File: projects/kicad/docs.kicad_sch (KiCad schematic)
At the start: 20 parts, among them J1 Micro_SD_Card, SW1 SW_PUSH, SW2 SW_PUSH, SW3 SW_PUSH, SW4 SW_PUSH, SW5 SW_PUSH, SW6 SW_PUSH, SW7 RotaryEncoder_Switch, U1 Pico, U2 LCD

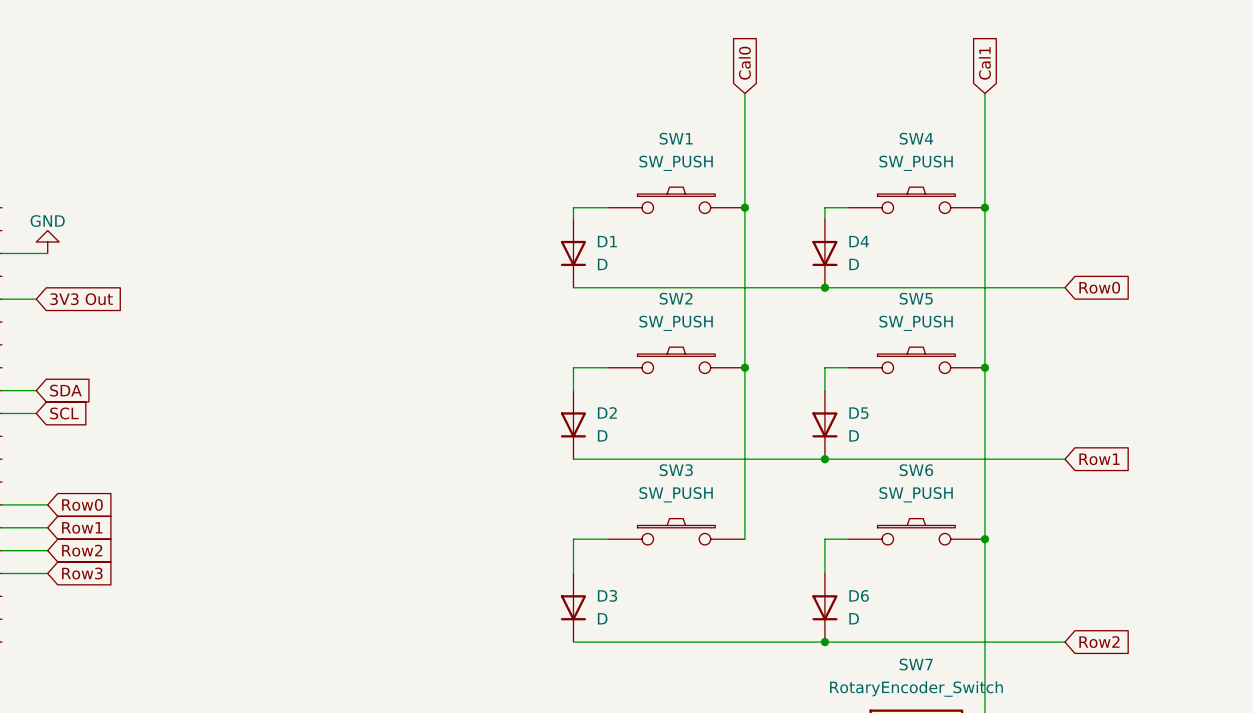
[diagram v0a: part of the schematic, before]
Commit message: Update_0122
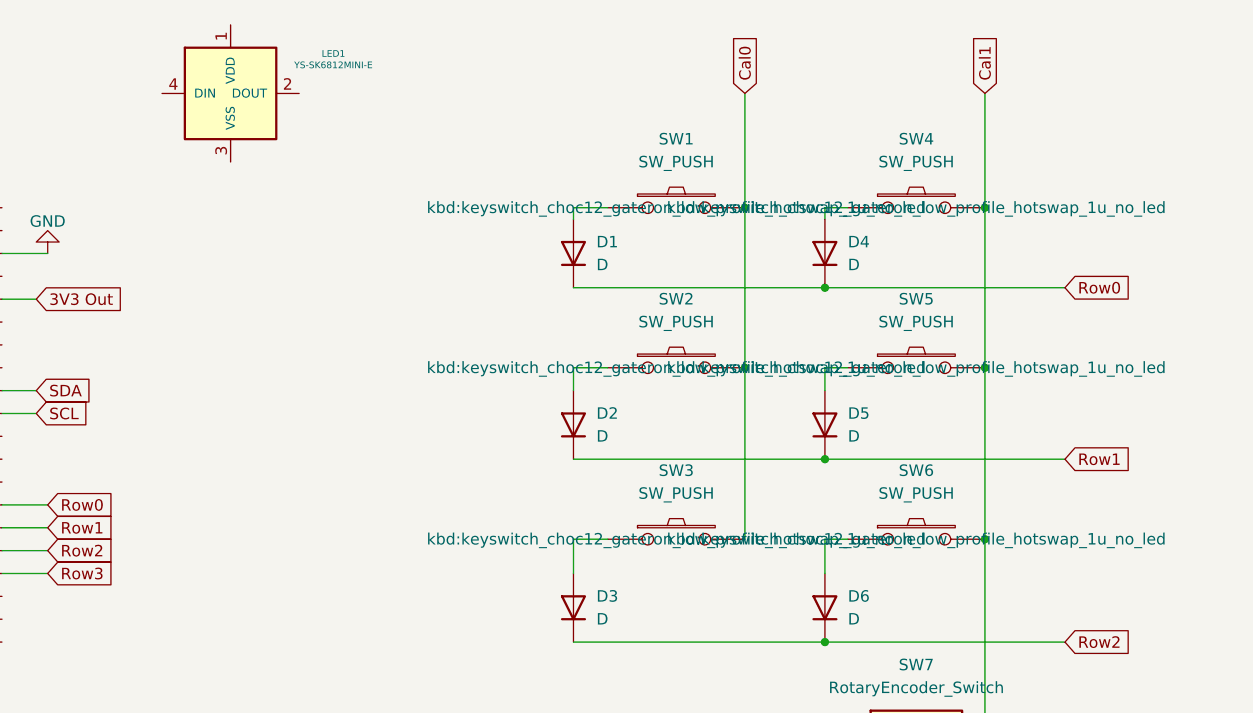
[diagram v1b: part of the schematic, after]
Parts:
- added LED1: YS-SK6812MINI-E, symbol kbd:YS-SK6812MINI-E
- D1, D2, D3, D4, D5, D6, D7: footprint (none) -> kbd_parts:D_SOD-123-Pretty
- SW1, SW2, SW3, SW4, SW5, SW6: footprint (none) -> kbd:keyswitch_choc12_gateron_low_profile_hotswap_1u_no_led
- SW7: footprint (none) -> Rotary_Encoder:RotaryEncoder_Bourns_Vertical_PEC12R-3x17F-Sxxxx
- U2: footprint (none) -> ST7789v_Library:ST7789V
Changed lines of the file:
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@@
 			)
 		)
-		(property "Footprint" ""
+		(property "Footprint" "kbd:keyswitch_choc12_gateron_low_profile_hotswap_1u_no_led"
 			(at 177.8 39.37 0)
 			(effects
@@
 			)
 		)
-		(property "Footprint" ""
+		(property "Footprint" "ST7789v_Library:ST7789V"
 			(at 153.67 123.19 0)
 			(effects
@@
 			)
 		)
-		(property "Footprint" ""
+		(property "Footprint" "kbd_parts:D_SOD-123-Pretty"
 			(at 139.7 83.82 0)
 			(effects
@@
 			)
 		)
-		(property "Footprint" ""
+		(property "Footprint" "kbd_parts:D_SOD-123-Pretty"
 			(at 167.64 63.5 0)
 			(effects
@@
 			)
 		)
-		(property "Footprint" ""
+		(property "Footprint" "kbd_parts:D_SOD-123-Pretty"
 			(at 139.7 44.45 0)
 			(effects
@@
 			)
 		)
-		(property "Footprint" ""
+		(property "Footprint" "kbd:keyswitch_choc12_gateron_low_profile_hotswap_1u_no_led"
 			(at 177.8 57.15 0)
 			(effects
@@
 			)
 		)
-		(property "Footprint" ""
+		(property "Footprint" "Rotary_Encoder:RotaryEncoder_Bourns_Vertical_PEC12R-3x17F-Sxxxx"
 			(at 173.99 96.266 0)
 			(effects
@@
 				(path "/eb9efe38-c1c1-4280-ba2b-08a47c3e2531"
 					(reference "SW7")
+					(unit 1)
+				)
+			)
+		)
+	)
+	(symbol
+		(lib_id "kbd:YS-SK6812MINI-E")
+		(at 101.6 26.67 0)
+		(unit 1)
+		(exclude_from_sim no)
+		(in_bom yes)
+		(on_board yes)
+		(dnp no)
+		(fields_autoplaced yes)
+		(property "Reference" "LED1"
+			(at 113.03 22.2565 0)
+			(effects
+				(font
+					(size 0.7366 0.7366)
+				)
+			)
+		)
+		(property "Value" "YS-SK6812MINI-E"
+			(at 113.03 23.5265 0)
+			(effects
+				(font
+					(size 0.7366 0.7366)
+				)
+			)
+		)
+		(property "Footprint" ""
+			(at 104.14 33.02 0)
+			(effects
+				(font
+					(size 1.27 1.27)
+				)
+				(hide yes)
+			)
+		)
+		(property "Datasheet" ""
+			(at 104.14 33.02 0)
+			(effects
+				(font
+					(size 1.27 1.27)
+				)
+				(hide yes)
+			)
+		)
+		(property "Description" ""
+			(at 101.6 26.67 0)
+			(effects
+				(font
+					(size 1.27 1.27)
+				)
+				(hide yes)
+			)
+		)
+		(pin "4"
+		)
+		(pin "2"
+		)
+		(pin "1"
+		)
+		(pin "3"
+		)
+		(instances
+			(project ""
+				(path "/eb9efe38-c1c1-4280-ba2b-08a47c3e2531"
+					(reference "LED1")
 					(unit 1)
 				)
@@
 			)
 		)
-		(property "Footprint" ""
+		(property "Footprint" "kbd_parts:D_SOD-123-Pretty"
 			(at 187.96 107.95 0)
 			(effects
@@
 			)
 		)
-		(property "Footprint" ""
+		(property "Footprint" "kbd_parts:D_SOD-123-Pretty"
 			(at 167.64 44.45 0)
 			(effects
@@
 			)
 		)
-		(property "Footprint" ""
+		(property "Footprint" "kbd_parts:D_SOD-123-Pretty"
 			(at 167.64 83.82 0)
 			(effects
@@
 			)
 		)
-		(property "Footprint" ""
+		(property "Footprint" "kbd:keyswitch_choc12_gateron_low_profile_hotswap_1u_no_led"
 			(at 151.13 76.2 0)
 			(effects
@@
 			)
 		)
-		(property "Footprint" ""
+		(property "Footprint" "kbd:keyswitch_choc12_gateron_low_profile_hotswap_1u_no_led"
 			(at 151.13 57.15 0)
 			(effects
@@
 			)
 		)
-		(property "Footprint" ""
+		(property "Footprint" "kbd:keyswitch_choc12_gateron_low_profile_hotswap_1u_no_led"
 			(at 151.13 39.37 0)
 			(effects
@@
 			)
 		)
-		(property "Footprint" ""
+		(property "Footprint" "kbd:keyswitch_choc12_gateron_low_profile_hotswap_1u_no_led"
 			(at 177.8 76.2 0)
 			(effects
@@
 			)
 		)
-		(property "Footprint" ""
+		(property "Footprint" "kbd_parts:D_SOD-123-Pretty"
 			(at 139.7 63.5 0)
 			(effects
